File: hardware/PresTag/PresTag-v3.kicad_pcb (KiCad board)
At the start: 2 copper layers, 17.2 x 9 mm, 20 parts, among them J201 CONN_02X04, J301 Conn_01x01, J302 Conn_01x01, J303 Conn_01x01, J304 Conn_01x01, J401 CONN_01X02, Q501 Q_NPN_BEC, U1 at25ex321D-UUN, U2 LPS27HHWTR, U302 stm32l431kc, U501 RV-3028-C7

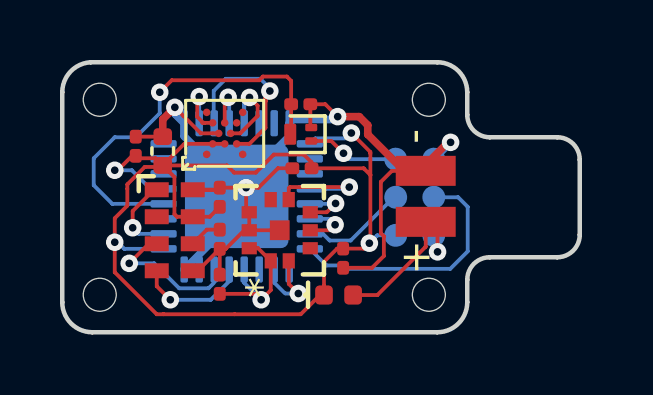
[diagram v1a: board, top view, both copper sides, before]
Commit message: revise prestag
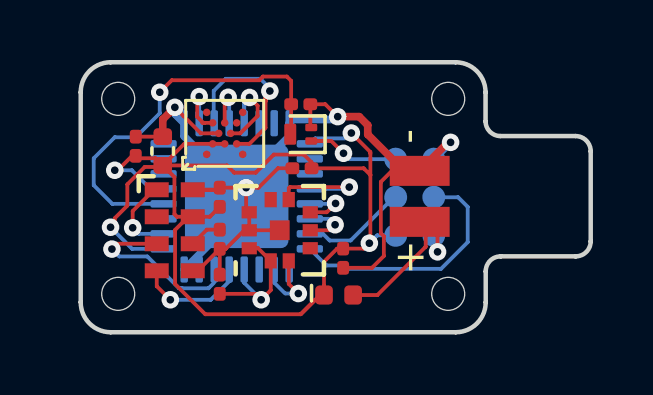
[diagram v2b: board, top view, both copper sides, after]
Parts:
- U2: footprint library:LPS27HHWTR -> lib_fp:LPS27HHWTR
- moved J401 0.20 mm to (151.2, 108.4)
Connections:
- U1 pad A1: (no net) -> unconnected-(U1-PadA1)
- U1 pad A5: (no net) -> unconnected-(U1-PadA5)
- U1 pad F4: (no net) -> unconnected-(U1-PadF4)
- U1 pad G1: (no net) -> unconnected-(U1-PadG1)
- U1 pad G5: (no net) -> unconnected-(U1-PadG5)
- U2 pad 3: (no net) -> unconnected-(U2-Pad3)
- U2 pad 7: (no net) -> unconnected-(U2-Pad7)
- U302 pad 14: (no net) -> unconnected-(U302-Pad14)
- U302 pad 15: (no net) -> unconnected-(U302-Pad15)
- U302 pad 18: (no net) -> unconnected-(U302-Pad18)
- U302 pad 19: (no net) -> unconnected-(U302-Pad19)
- U302 pad 25: (no net) -> unconnected-(U302-Pad25)
- U302 pad 27: (no net) -> unconnected-(U302-Pad27)
- U302 pad 3: (no net) -> unconnected-(U302-Pad3)
- U302 pad 6: (no net) -> unconnected-(U302-Pad6)
- U302 pad 7: (no net) -> unconnected-(U302-Pad7)
- U302 pad 8: (no net) -> unconnected-(U302-Pad8)
- U501 pad 2: (no net) -> unconnected-(U501-Pad2)
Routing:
- net /SCL: track 4.44 -> 5.74 mm
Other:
- board size 17.2 x 9 mm -> 17 x 9 mm
- board text added: "PresTag v4"
- board text removed: "PresTag v3"
